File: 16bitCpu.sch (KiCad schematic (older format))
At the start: 0 parts

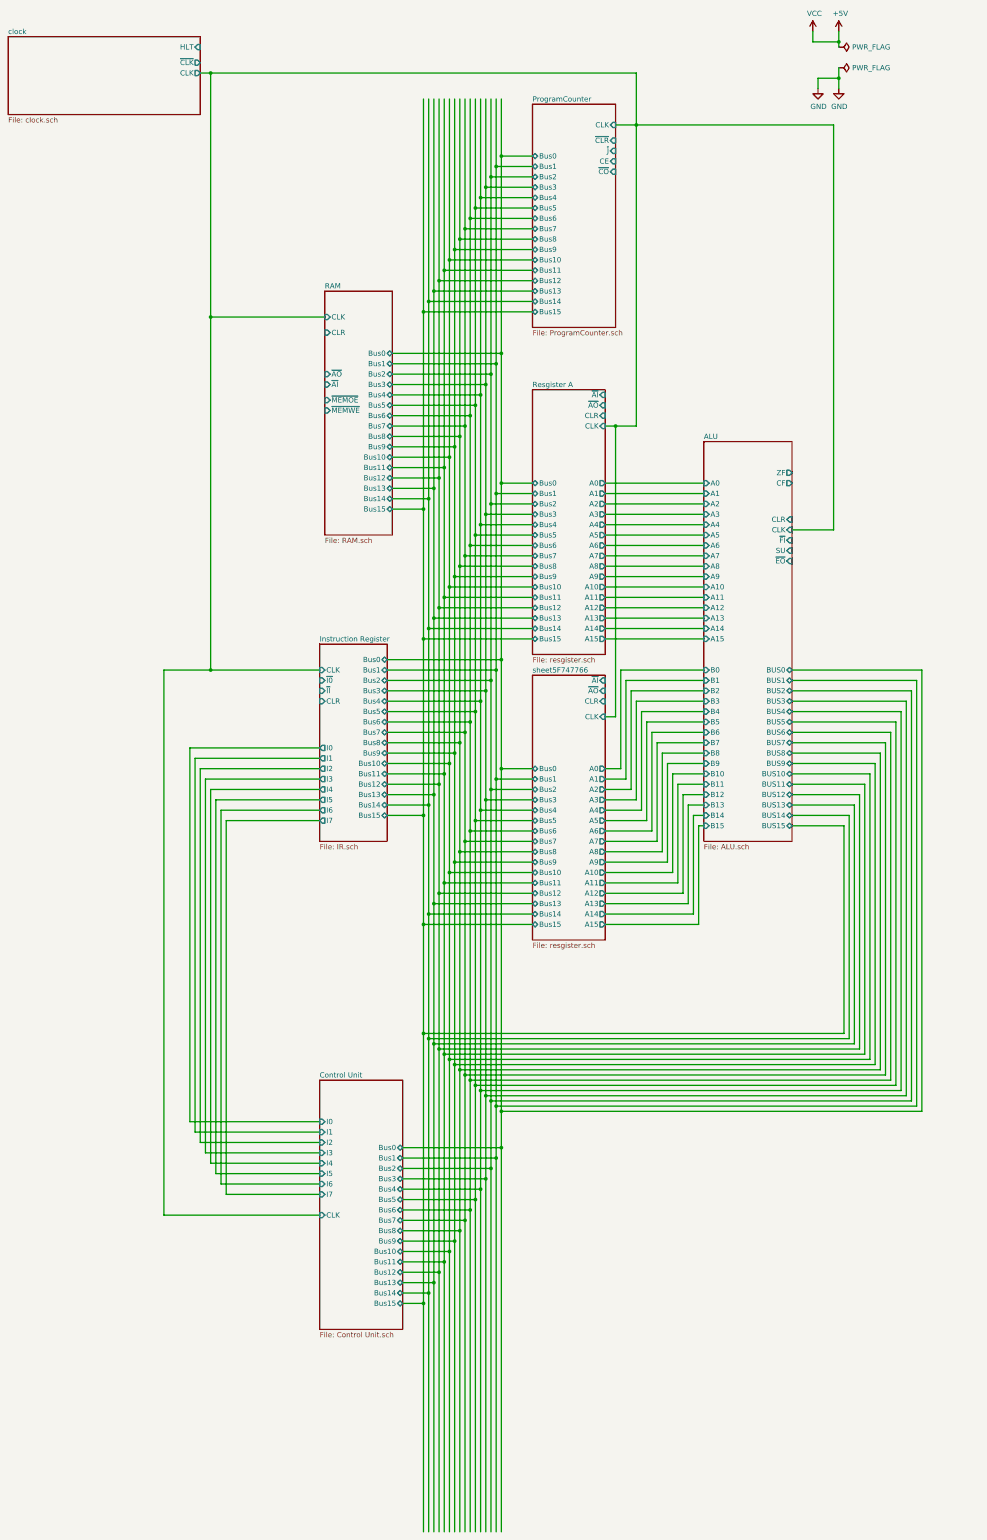
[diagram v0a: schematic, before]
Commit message: made the CU , need to change the IR
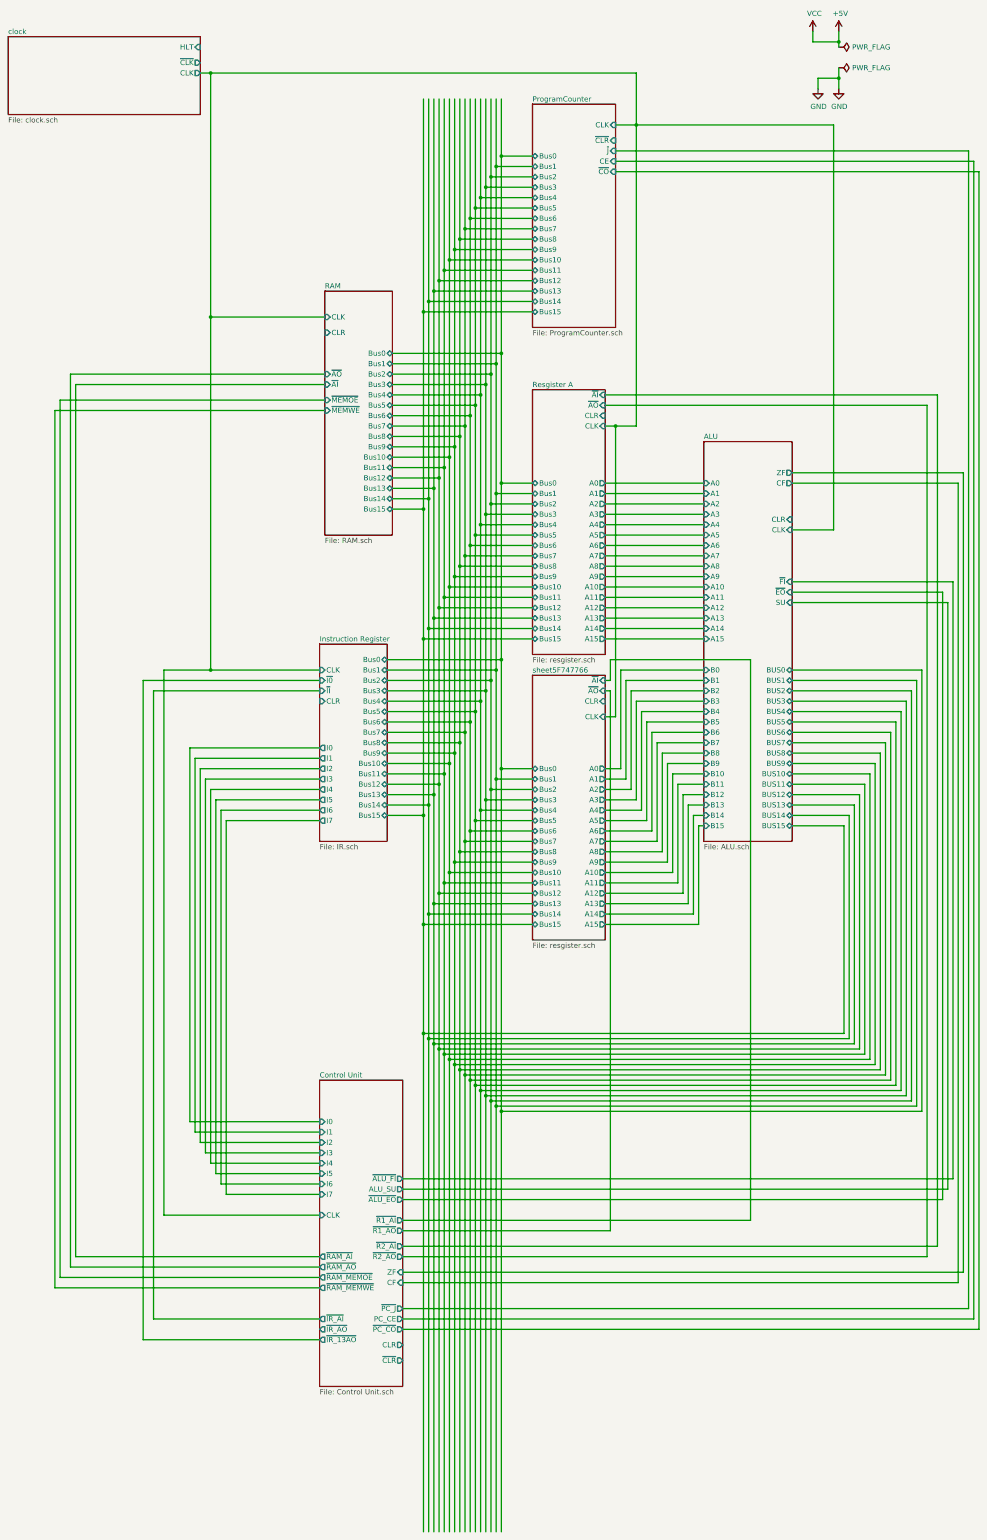
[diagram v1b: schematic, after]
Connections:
- wire segments 387 -> 411
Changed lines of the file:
@@
 F16 "A14" I L 8050 6950 50
 F17 "A15" I L 8050 7050 50
-F18 "SU" I R 8900 6200 50
+F18 "SU" I R 8900 6700 50
 F19 "B15" I L 8050 8850 50
 F20 "B14" I L 8050 8750 50
@@
 F33 "B1" I L 8050 7450 50
 F34 "B0" I L 8050 7350 50
-F35 "~EO" I R 8900 6300 50
+F35 "~EO" I R 8900 6600 50
 F36 "BUS0" T R 8900 7350 50
 F37 "BUS1" T R 8900 7450 50
@@
 F50 "BUS14" T R 8900 8750 50
 F51 "BUS15" T R 8900 8850 50
-F52 "~FI" I R 8900 6100 50
+F52 "~FI" I R 8900 6500 50
 F53 "CLK" I R 8900 6000 50
 F54 "CLR" I R 8900 5900 50
@@
 	7100 9400 7800 9400
 Wire Wire Line
-	7800 9400 7800 8450
-Wire Wire Line
 	7800 8450 8050 8450
 Wire Wire Line
@@
 Wire Wire Line
 	7250 7350 8050 7350
-Wire Wire Line
-	7300 7450 8050 7450
 Wire Wire Line
 	7350 7550 8050 7550
@@
 Wire Wire Line
 	7400 2100 7400 1600
-Wire Wire Line
-	6050 11550 6050 12050
-Wire Wire Line
-	6000 11500 6000 12150
-Wire Wire Line
-	5950 11450 5950 12250
-Wire Wire Line
-	5900 11400 5900 12350
-Wire Wire Line
-	5750 11250 5750 12650
-Wire Wire Line
-	5700 11200 5700 12750
-Wire Wire Line
-	5650 11150 5650 12850
-Wire Wire Line
-	5600 11100 5600 12950
-Wire Wire Line
-	5550 11050 5550 13050
-Wire Wire Line
-	5500 11000 5500 13150
-Wire Wire Line
-	5450 10950 5450 13250
-Wire Wire Line
-	5400 10900 5400 13350
 Wire Wire Line
 	5000 7250 6100 7250
@@
 	3300 3950 4400 3950
 Wire Wire Line
-	6100 11600 6100 11950
-Wire Wire Line
-	5350 10850 5350 13450
-Wire Wire Line
 	5350 9800 6400 9800
 Wire Wire Line
 	5450 9600 5450 10950
-Wire Wire Line
-	5150 11950 6100 11950
-Connection ~ 6100 11950
-Wire Wire Line
-	6100 11950 6100 15650
-Wire Wire Line
-	5150 12050 6050 12050
-Connection ~ 6050 12050
-Wire Wire Line
-	6050 12050 6050 15650
-Wire Wire Line
-	5150 12150 6000 12150
-Connection ~ 6000 12150
-Wire Wire Line
-	6000 12150 6000 15650
-Wire Wire Line
-	5150 12250 5950 12250
-Connection ~ 5950 12250
-Wire Wire Line
-	5950 12250 5950 15650
-Wire Wire Line
-	5150 12350 5900 12350
-Connection ~ 5900 12350
-Wire Wire Line
-	5900 12350 5900 15650
-Wire Wire Line
-	5150 12450 5850 12450
-Wire Wire Line
-	5850 11350 5850 12450
-Connection ~ 5850 12450
-Wire Wire Line
-	5850 12450 5850 15650
-Wire Wire Line
-	5150 12550 5800 12550
-Wire Wire Line
-	5800 11300 5800 12550
-Connection ~ 5800 12550
-Wire Wire Line
-	5800 12550 5800 15650
-Wire Wire Line
-	5150 12650 5750 12650
-Connection ~ 5750 12650
-Wire Wire Line
-	5750 12650 5750 15650
-Wire Wire Line
-	5150 12750 5700 12750
-Connection ~ 5700 12750
-Wire Wire Line
-	5700 12750 5700 15650
-Wire Wire Line
-	5150 12850 5650 12850
-Connection ~ 5650 12850
-Wire Wire Line
-	5650 12850 5650 15650
-Wire Wire Line
-	5150 12950 5600 12950
-Connection ~ 5600 12950
-Wire Wire Line
-	5600 12950 5600 15650
-Wire Wire Line
-	5150 13050 5550 13050
-Connection ~ 5550 13050
-Wire Wire Line
-	5550 13050 5550 15650
-Wire Wire Line
-	5150 13150 5500 13150
-Connection ~ 5500 13150
-Wire Wire Line
-	5500 13150 5500 15650
-Wire Wire Line
-	5150 13250 5450 13250
-Connection ~ 5450 13250
-Wire Wire Line
-	5450 13250 5450 15650
-Wire Wire Line
-	5150 13350 5400 13350
-Connection ~ 5400 13350
-Wire Wire Line
-	5400 13350 5400 15650
-Wire Wire Line
-	5150 13450 5350 13450
-Connection ~ 5350 13450
-Wire Wire Line
-	5350 13450 5350 15650
-$Sheet
-S 4350 11300 800  2400
-U 5FD099BF
-F0 "Control Unit" 50
-F1 "Control Unit.sch" 50
-F2 "Bus1" T R 5150 12050 50
-F3 "Bus0" T R 5150 11950 50
-F4 "Bus2" T R 5150 12150 50
-F5 "Bus3" T R 5150 12250 50
-F6 "Bus4" T R 5150 12350 50
-F7 "Bus5" T R 5150 12450 50
-F8 "Bus6" T R 5150 12550 50
-F9 "Bus7" T R 5150 12650 50
-F10 "Bus9" T R 5150 12850 50
-F11 "Bus10" T R 5150 12950 50
-F12 "Bus11" T R 5150 13050 50
-F13 "Bus12" T R 5150 13150 50
-F14 "Bus13" T R 5150 13250 50
-F15 "Bus14" T R 5150 13350 50
-F16 "Bus15" T R 5150 13450 50
-F17 "Bus8" T R 5150 12750 50
-F18 "I1" I L 4350 11800 50
-F19 "I0" I L 4350 11700 50
-F20 "I2" I L 4350 11900 50
-F21 "I3" I L 4350 12000 50
-F22 "I4" I L 4350 12100 50
-F23 "I5" I L 4350 12200 50
-F24 "I6" I L 4350 12300 50
-F25 "I7" I L 4350 12400 50
-F26 "CLK" I L 4350 12600 50
-$EndSheet
 Wire Wire Line
 	3100 8100 3100 11700
@@
 Wire Wire Line
 	9300 6000 8900 6000
+$Sheet
+S 4350 11300 800  2950
+U 5FD099BF
+F0 "Control Unit" 50
+F1 "Control Unit.sch" 50
+F2 "I1" I L 4350 11800 50
+F3 "I0" I L 4350 11700 50
+F4 "I2" I L 4350 11900 50
+F5 "I3" I L 4350 12000 50
+F6 "I4" I L 4350 12100 50
+F7 "I5" I L 4350 12200 50
+F8 "I6" I L 4350 12300 50
+F9 "I7" I L 4350 12400 50
+F10 "CLK" I L 4350 12600 50
+F11 "ZF" I R 5150 13150 50
+F12 "CF" I R 5150 13250 50
+F13 "~ALU_FI" O R 5150 12250 50
+F14 "ALU_SU" O R 5150 12350 50
+F15 "~ALU_EO" O R 5150 12450 50
+F16 "~R1_AI" O R 5150 12650 50
+F17 "~R1_AO" O R 5150 12750 50
+F18 "~R2_AI" O R 5150 12900 50
+F19 "~R2_AO" O R 5150 13000 50
+F20 "~RAM_AI" O L 4350 13000 50
+F21 "~RAM_AO" O L 4350 13100 50
+F22 "~RAM_MEMOE" O L 4350 13200 50
+F23 "~RAM_MEMWE" O L 4350 13300 50
+F24 "~IR_AI" O L 4350 13600 50
+F25 "~IR_AO" O L 4350 13700 50
+F26 "~IR_13AO" O L 4350 13800 50
+F27 "~PC_J" O R 5150 13500 50
+F28 "PC_CE" O R 5150 13600 50
+F29 "~PC_CO" O R 5150 13700 50
+F30 "CLR" O R 5150 13850 50
+F31 "~CLR" O R 5150 14000 50
+$EndSheet
+Wire Wire Line
+	6100 11600 6100 15650
+Wire Wire Line
+	6050 11550 6050 15650
+Wire Wire Line
+	6000 11500 6000 15650
+Wire Wire Line
+	5950 11450 5950 15650
+Wire Wire Line
+	5900 11400 5900 15650
+Wire Wire Line
+	5850 11350 5850 15650
+Wire Wire Line
+	5800 11300 5800 15650
+Wire Wire Line
+	5750 11250 5750 15650
+Wire Wire Line
+	5700 11200 5700 15650
+Wire Wire Line
+	5650 11150 5650 15650
+Wire Wire Line
+	5600 11100 5600 15650
+Wire Wire Line
+	5550 11050 5550 15650
+Wire Wire Line
+	5500 11000 5500 15650
+Wire Wire Line
+	5450 10950 5450 15650
+Wire Wire Line
+	5400 10900 5400 15650
+Wire Wire Line
+	5350 10850 5350 15650
+Wire Wire Line
+	8900 5450 10550 5450
+Wire Wire Line
+	10550 5450 10550 13150
+Wire Wire Line
+	10550 13150 5150 13150
+Wire Wire Line
+	8900 5550 10500 5550
+Wire Wire Line
+	10500 5550 10500 13250
+Wire Wire Line
+	10500 13250 5150 13250
+Wire Wire Line
+	5150 12250 10450 12250
+Wire Wire Line
+	10450 12250 10450 6500
+Wire Wire Line
+	10450 6500 8900 6500
+Wire Wire Line
+	5150 12350 10400 12350
+Wire Wire Line
+	10400 12350 10400 6700
+Wire Wire Line
+	10400 6700 8900 6700
+Wire Wire Line
+	5150 12450 10350 12450
+Wire Wire Line
+	10350 12450 10350 6600
+Wire Wire Line
+	10350 6600 8900 6600
+Wire Wire Line
+	7300 7450 8050 7450
+Wire Wire Line
+	7100 7450 7150 7450
+Wire Wire Line
+	7150 7450 7150 7250
+Wire Wire Line
+	7150 7250 8500 7250
+Wire Wire Line
+	8500 7250 8500 12650
+Wire Wire Line
+	8500 12650 5150 12650
+Wire Wire Line
+	5150 12750 7150 12750
+Wire Wire Line
+	7150 12750 7150 7550
+Wire Wire Line
+	7150 7550 7100 7550
+Wire Wire Line
+	7800 9400 7800 8450
+Wire Wire Line
+	5150 12900 10300 12900
+Wire Wire Line
+	10300 12900 10300 4700
+Wire Wire Line
+	10300 4700 7100 4700
+Wire Wire Line
+	5150 13000 10200 13000
+Wire Wire Line
+	10200 13000 10200 4800
+Wire Wire Line
+	10200 4800 7100 4800
+Wire Wire Line
+	5150 13500 10600 13500
+Wire Wire Line
+	10600 13500 10600 2350
+Wire Wire Line
+	10600 2350 7200 2350
+Wire Wire Line
+	5150 13600 10650 13600
+Wire Wire Line
+	10650 13600 10650 2450
+Wire Wire Line
+	10650 2450 7200 2450
+Wire Wire Line
+	5150 13700 10700 13700
+Wire Wire Line
+	10700 13700 10700 2550
+Wire Wire Line
+	10700 2550 7200 2550
+Wire Wire Line
+	4350 13000 2000 13000
+Wire Wire Line
+	2000 13000 2000 4600
+Wire Wire Line
+	2000 4600 4400 4600
+Wire Wire Line
+	4350 13100 1950 13100
+Wire Wire Line
+	1950 13100 1950 4500
+Wire Wire Line
+	1950 4500 4400 4500
+Wire Wire Line
+	4350 13200 1850 13200
+Wire Wire Line
+	1850 13200 1850 4750
+Wire Wire Line
+	1850 4750 4400 4750
+Wire Wire Line
+	4350 13300 1800 13300
+Wire Wire Line
+	1800 13300 1800 4850
+Wire Wire Line
+	1800 4850 4400 4850
+Wire Wire Line
+	4350 13600 2750 13600
+Wire Wire Line
+	2750 13600 2750 7550
+Wire Wire Line
+	2750 7550 4350 7550
+Wire Wire Line
+	2650 7450 4350 7450
+Wire Wire Line
+	4350 13800 2650 13800
+Wire Wire Line
+	2650 7450 2650 13800
 $EndSCHEMATC
